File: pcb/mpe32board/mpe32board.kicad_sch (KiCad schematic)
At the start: 37 parts, among them J1 Conn_ST_STDC14, J2 USB_C_Receptacle_USB2.0_16P, SW1 SW_Push, SW2 SW_Push, U10 W9812G6KH-75, U2 USBLC6-2P6, U3 AMS1117-3.3, U9 STM32H743IITx

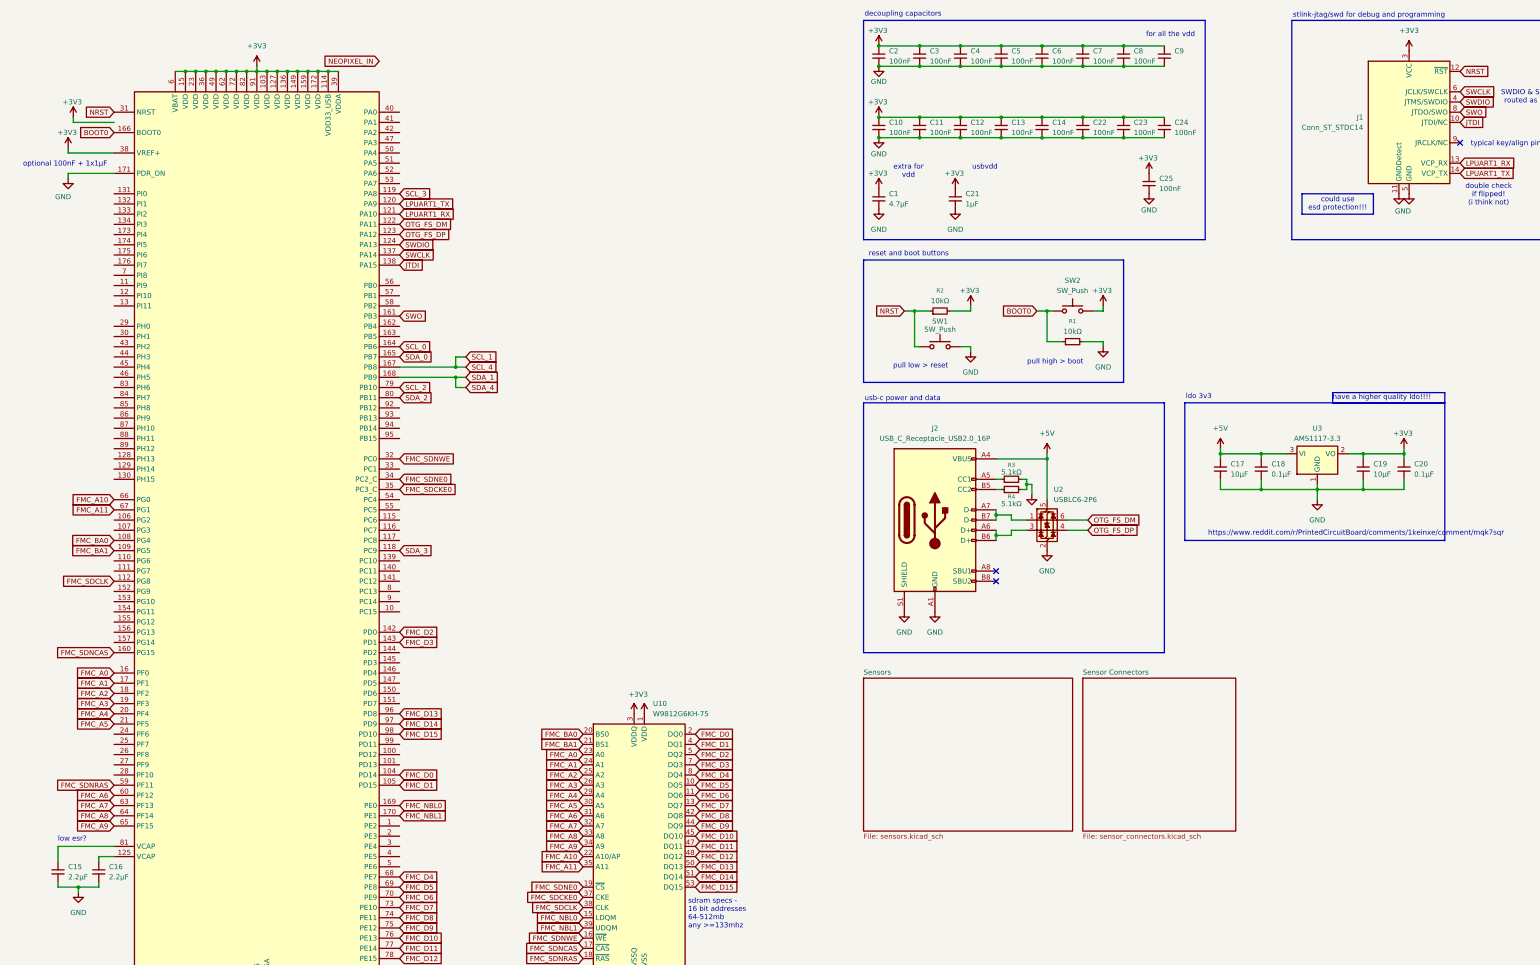
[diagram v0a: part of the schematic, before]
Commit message: codec
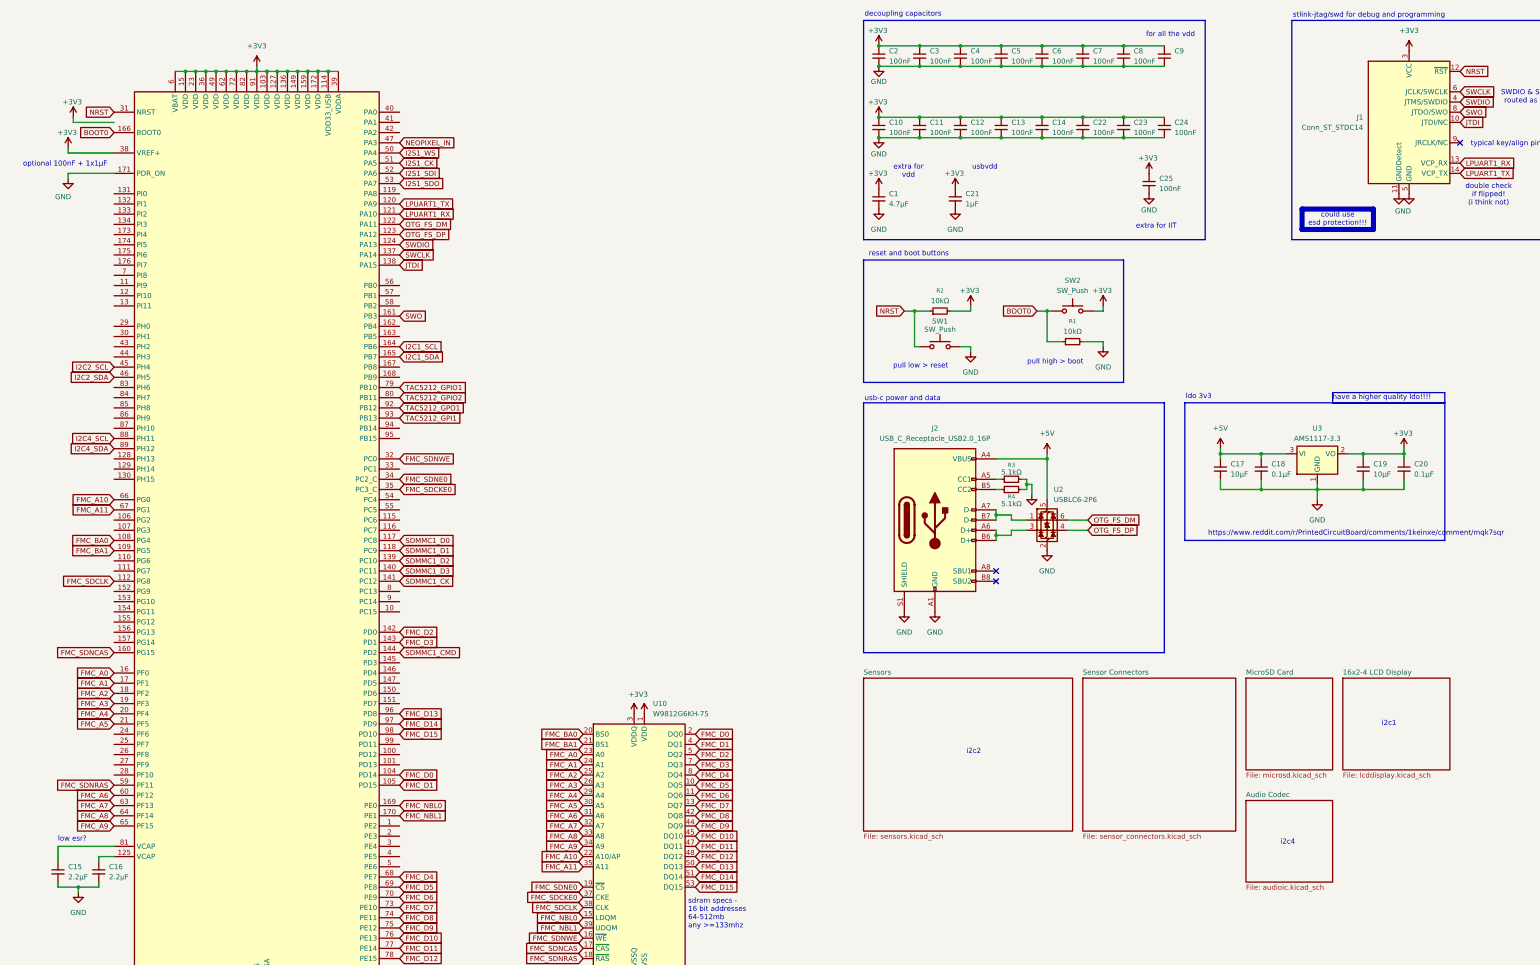
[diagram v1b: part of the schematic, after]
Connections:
- net NEOPIXEL_IN: now also U9.47 (PA3)
- net SDMMC1_D0: now reaches U9.117 (PC8)
- net SDMMC1_D2: now reaches U9.139 (PC10)
- net SDMMC1_D3: now reaches U9.140 (PC11)
- net SDMMC1_CK: now reaches U9.141 (PC12)
- net SDMMC1_CMD: now reaches U9.144 (PD2)
- net I2C2_SCL: now reaches U9.45 (PH4)
- net I2C2_SDA: now reaches U9.46 (PH5)
- net I2S1_WS: now reaches U9.50 (PA4)
- net I2S1_CK: now reaches U9.51 (PA5)
- net I2S1_SDI: now reaches U9.52 (PA6)
- net I2S1_SDO: now reaches U9.53 (PA7)
- net I2C4_SCL: now reaches U9.88 (PH11)
- net I2C4_SDA: now reaches U9.89 (PH12)
- net TAC5212_GPO1: now reaches U9.92 (PB12)
- net TAC5212_GPI1: now reaches U9.93 (PB13)
- net SCL_0 renamed I2C1_SCL
- net SCL_1: no longer names the net of U9.167 (PB8)
- net SCL_2 renamed TAC5212_GPIO1
- net SCL_3: no longer names the net of U9.119 (PA8)
- net SDA_0 renamed I2C1_SDA
- net SDA_1: no longer names the net of U9.168 (PB9)
- net SDA_2 renamed TAC5212_GPIO2
- net SDA_3 renamed SDMMC1_D1
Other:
- added sheet 16x2-4 LCD Display (lcddisplay.kicad_sch)
- added sheet Audio Codec (audioic.kicad_sch)
- added sheet MicroSD Card (microsd.kicad_sch)
- note added: "extra for IIT"
- note added: "i2c1"
- note added: "i2c2"
- note added: "i2c4"

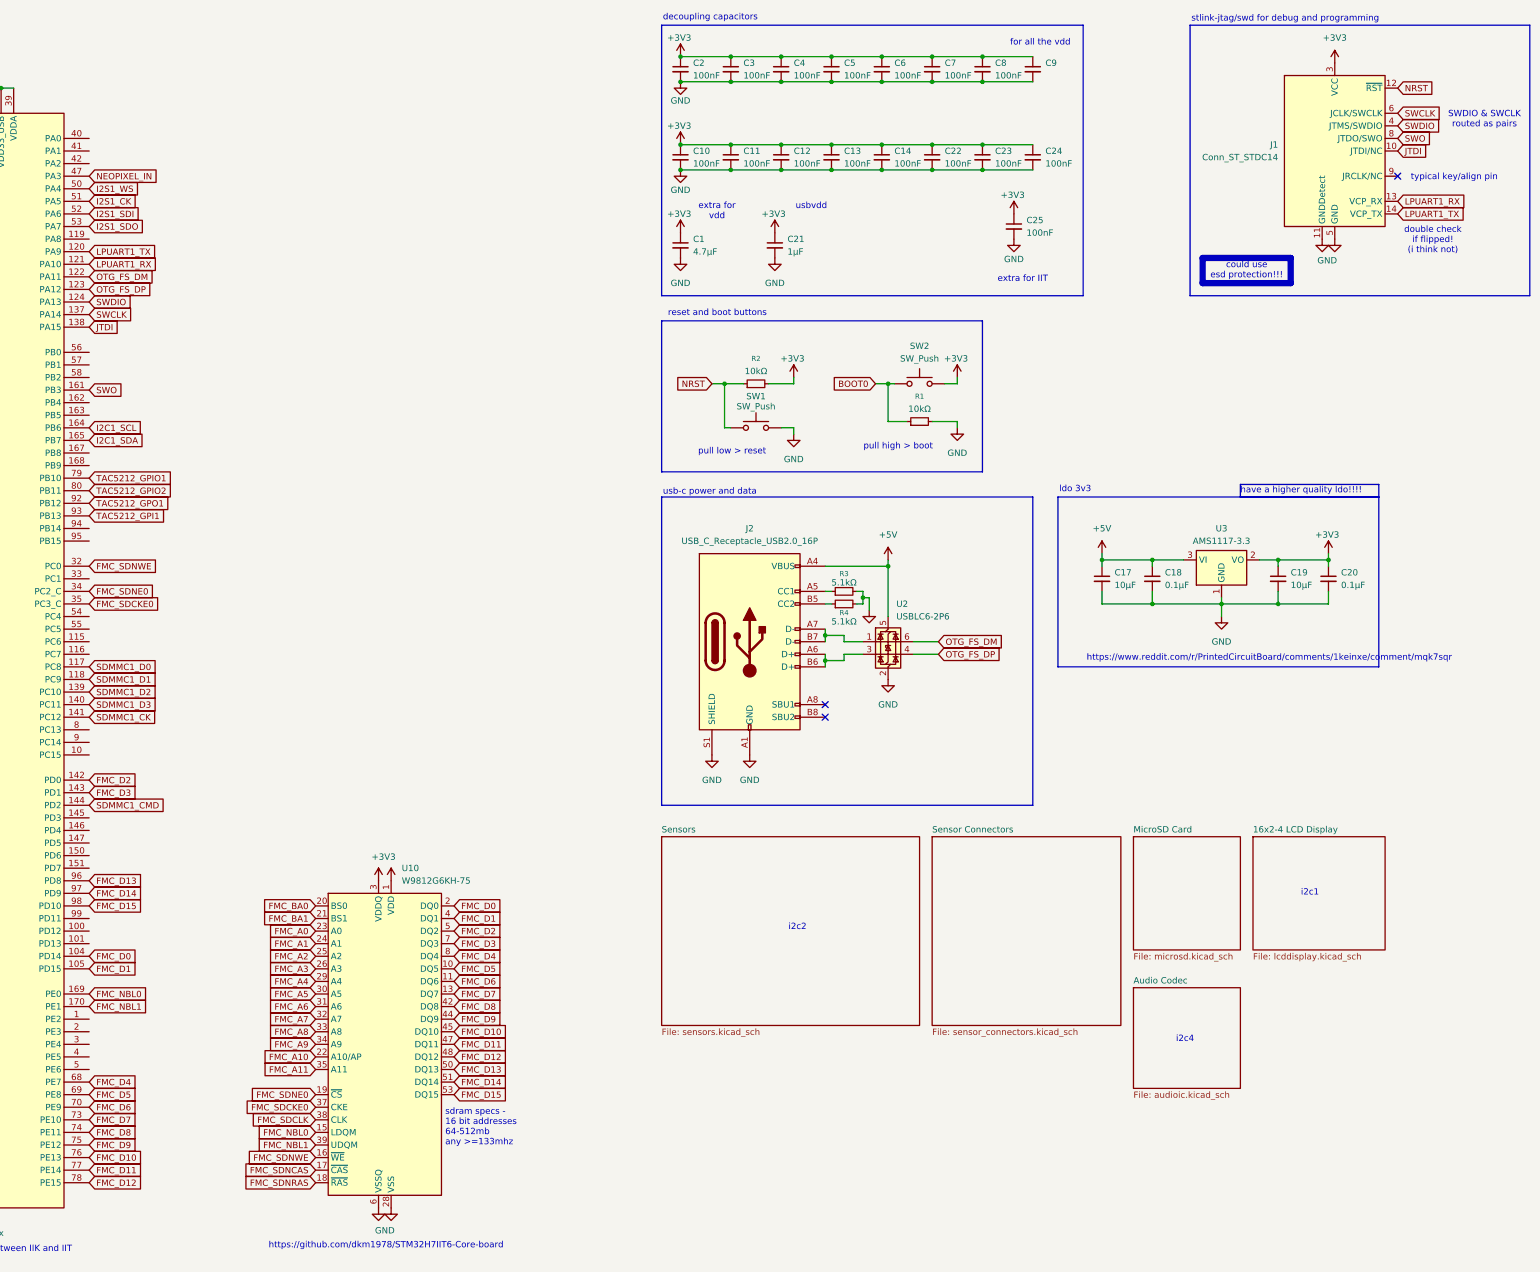
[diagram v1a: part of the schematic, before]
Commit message: layout stuff
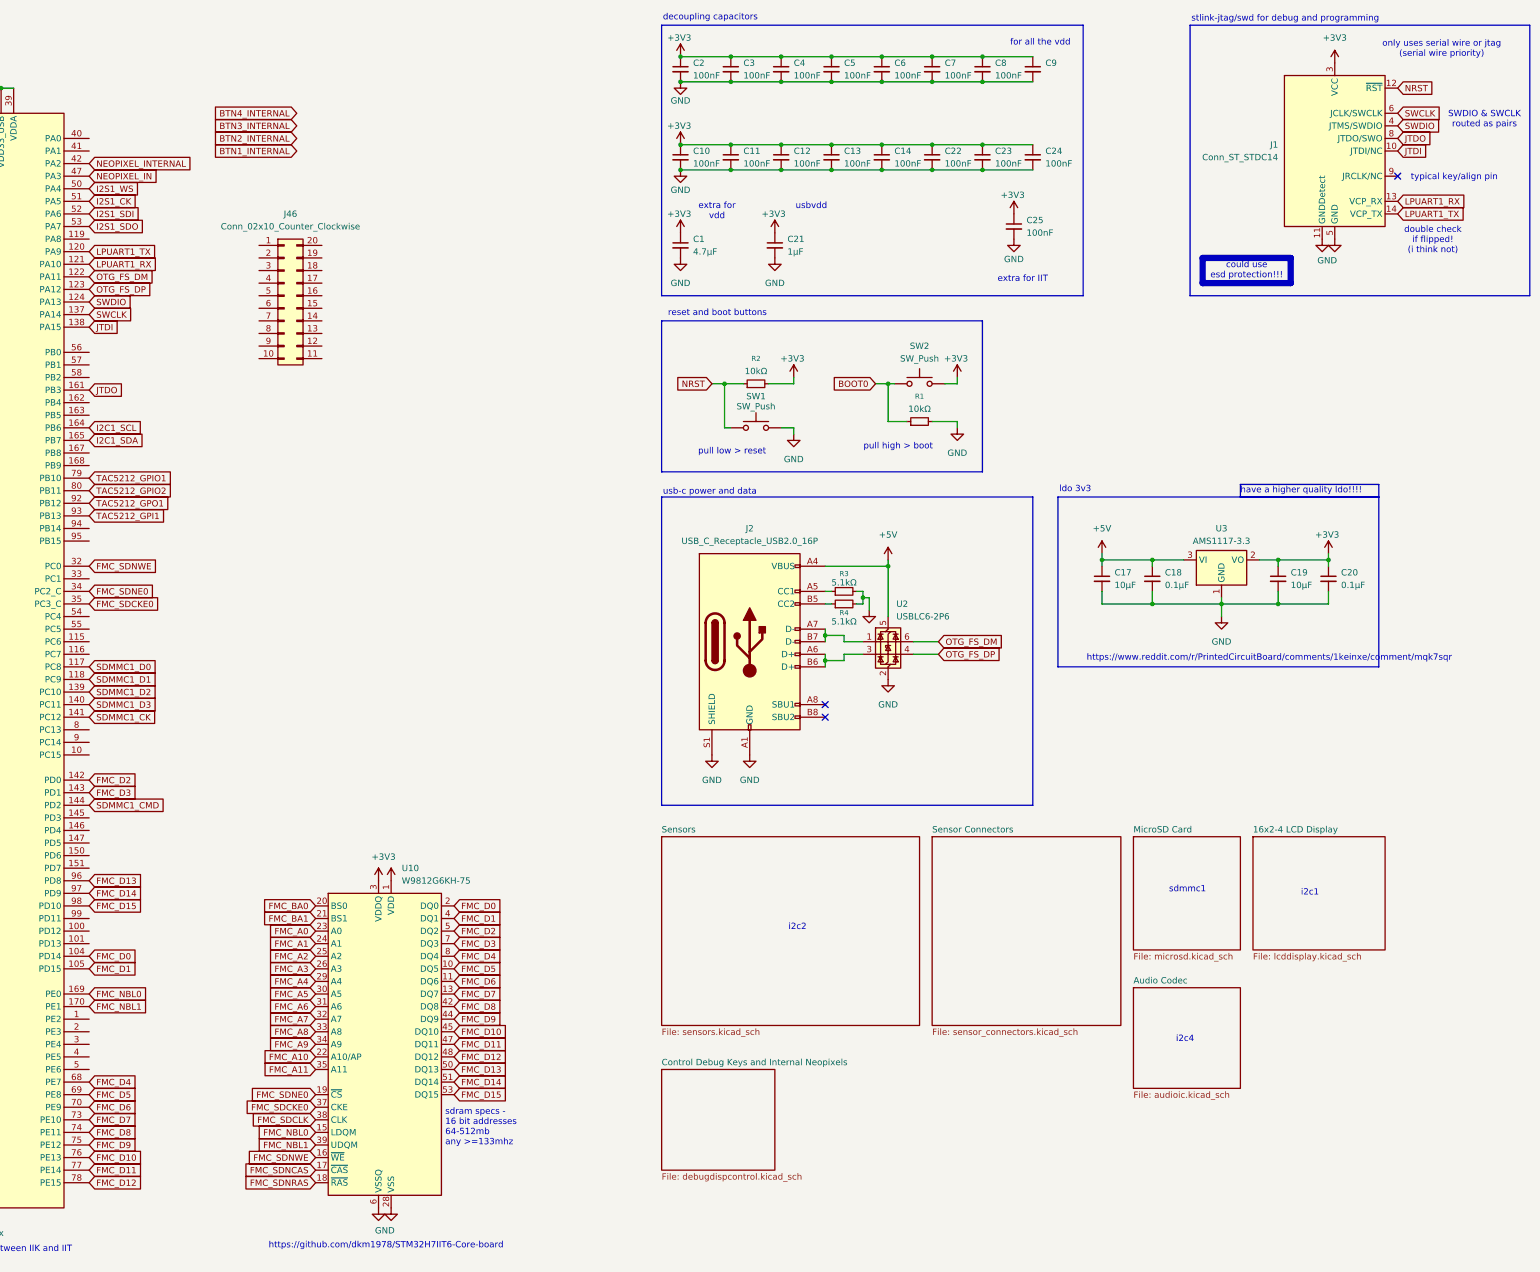
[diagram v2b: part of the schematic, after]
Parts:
- added J46: Conn_02x10_Counter_Clockwise, Connector_PinHeader_2.54mm:PinHeader_2x10_P2.54mm_Vertical, symbol Connector_Generic:Conn_02x10_Counter_Clockwise
- C1, C10, C11, C12, C13, C14, C15, C16, C17, C18, C19, C2, C20, C21, C22, C23, C24, C25, C3, C4, C5, C6, C7, C8, C9: footprint (none) -> Capacitor_SMD:C_0603_1608Metric
- J2: footprint (none) -> Connector_USB:USB_C_Receptacle_GCT_USB4105-xx-A_16P_TopMnt_Horizontal
- R1, R2, R3, R4: footprint (none) -> Resistor_SMD:R_0603_1608Metric
- SW1, SW2: footprint (none) -> Button_Switch_THT:SW_PUSH_6mm
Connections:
- net NEOPIXEL_INTERNAL: now reaches U9.42 (PA2)
- net SWO renamed JTDO
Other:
- added sheet Control Debug Keys and Internal Neopixels (debugdispcontrol.kicad_sch)
- note added: "only uses serial wire or jtag (serial wire priority)"
- note added: "sdmmc1"
